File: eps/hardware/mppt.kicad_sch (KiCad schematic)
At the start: 16 parts, among them U2 LTC3130-1

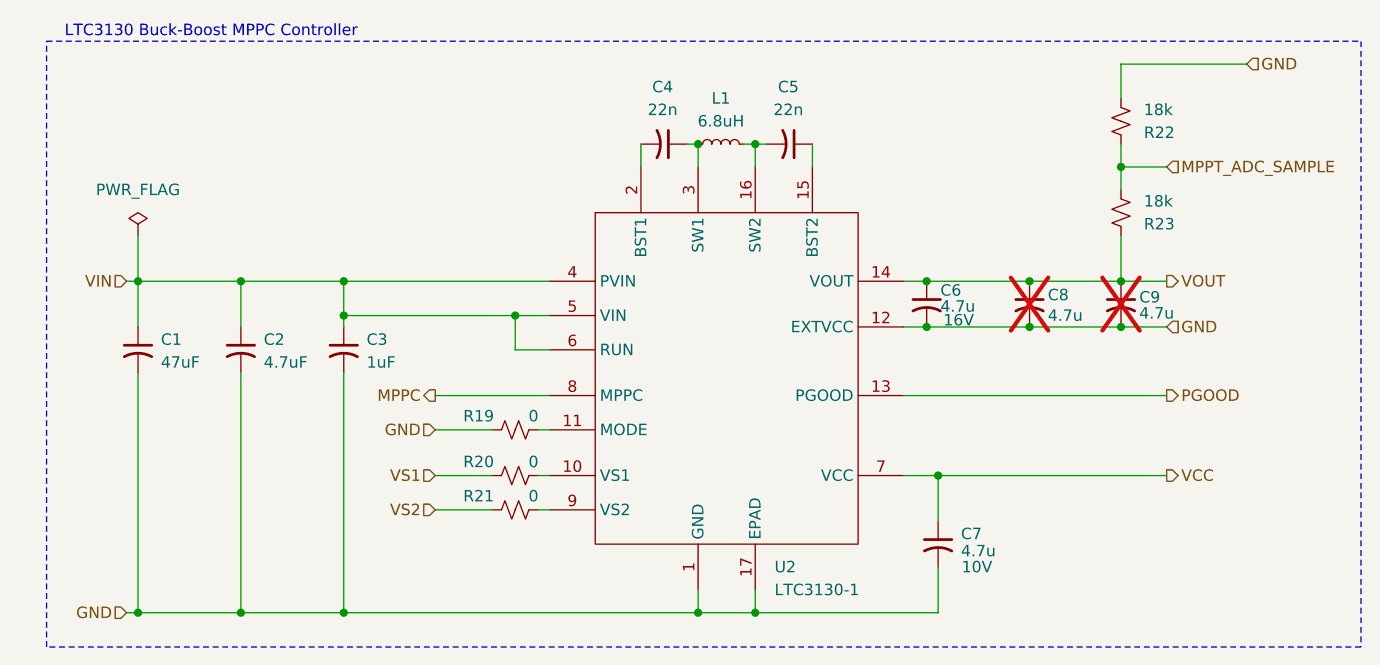
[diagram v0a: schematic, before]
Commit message: netlist fixes
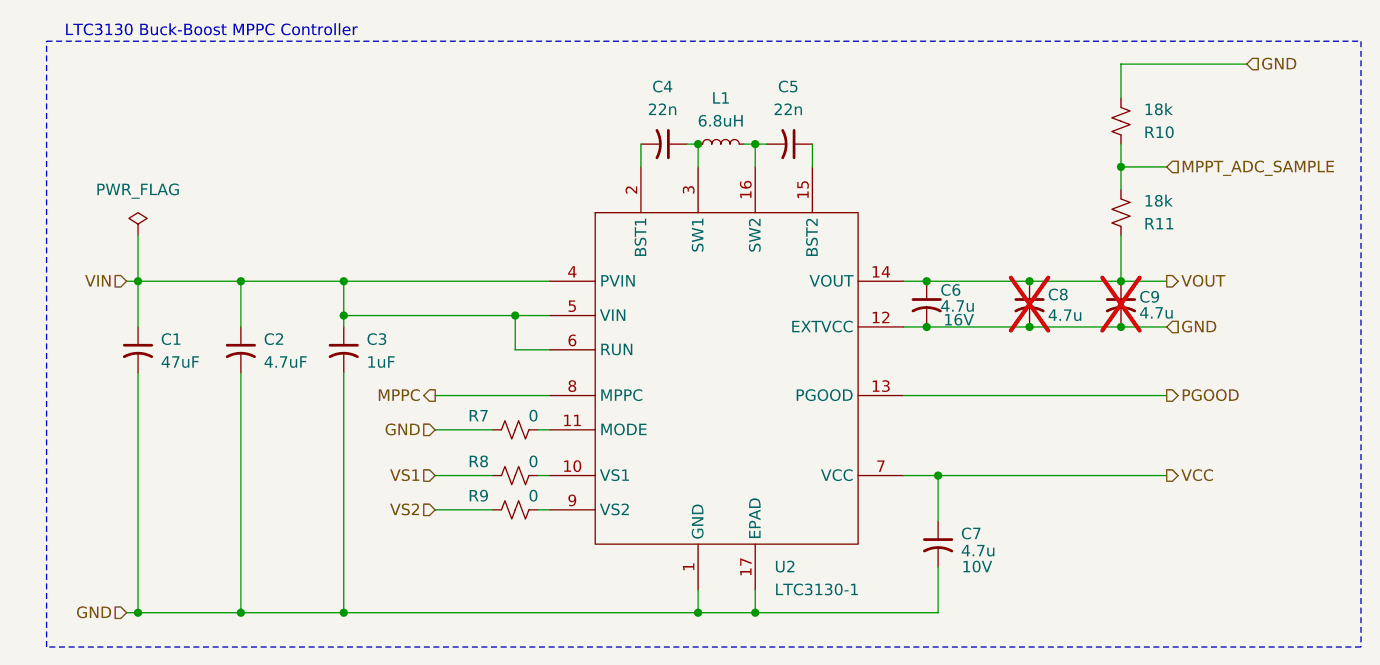
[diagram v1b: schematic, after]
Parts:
- renumbered R22 to R10, R23 to R11, R19 to R7, R20 to R8, R21 to R9
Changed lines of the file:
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@@
 		(on_board yes)
 		(dnp no)
-		(property "Reference" "R23"
+		(property "Reference" "R11"
 			(at 135.89 35.5601 0)
 			(effects
@@
 			(project "eps"
 				(path "/9e0ae2e7-d4be-41b4-8312-0d2aceea2180/fa2efaa0-4907-4b3e-94ec-ef462aa79480"
-					(reference "R23")
+					(reference "R11")
 					(unit 1)
 				)
@@
 		(on_board yes)
 		(dnp no)
-		(property "Reference" "R22"
+		(property "Reference" "R10"
 			(at 135.89 25.4001 0)
 			(effects
@@
 			(project "eps"
 				(path "/9e0ae2e7-d4be-41b4-8312-0d2aceea2180/fa2efaa0-4907-4b3e-94ec-ef462aa79480"
-					(reference "R22")
+					(reference "R10")
 					(unit 1)
 				)
@@
 		(on_board yes)
 		(dnp no)
-		(property "Reference" "R20"
+		(property "Reference" "R8"
 			(at 61.976 61.976 90)
 			(effects
@@
 			(project ""
 				(path "/9e0ae2e7-d4be-41b4-8312-0d2aceea2180/fa2efaa0-4907-4b3e-94ec-ef462aa79480"
-					(reference "R20")
+					(reference "R8")
 					(unit 1)
 				)
@@
 		(on_board yes)
 		(dnp no)
-		(property "Reference" "R21"
+		(property "Reference" "R9"
 			(at 61.976 65.786 90)
 			(effects
@@
 			(project "eps"
 				(path "/9e0ae2e7-d4be-41b4-8312-0d2aceea2180/fa2efaa0-4907-4b3e-94ec-ef462aa79480"
-					(reference "R21")
+					(reference "R9")
 					(unit 1)
 				)
@@
 		(on_board yes)
 		(dnp no)
-		(property "Reference" "R19"
+		(property "Reference" "R7"
 			(at 61.976 56.896 90)
 			(effects
@@
 			(project "eps"
 				(path "/9e0ae2e7-d4be-41b4-8312-0d2aceea2180/fa2efaa0-4907-4b3e-94ec-ef462aa79480"
-					(reference "R19")
+					(reference "R7")
 					(unit 1)
 				)
@@
 		(dnp no)
 		(fields_autoplaced yes)
-		(property "Reference" "#FLG02"
+		(property "Reference" "#FLG03"
 			(at 24.13 34.925 0)
 			(effects
@@
 			(project "eps"
 				(path "/9e0ae2e7-d4be-41b4-8312-0d2aceea2180/fa2efaa0-4907-4b3e-94ec-ef462aa79480"
-					(reference "#FLG02")
-					(unit 1)
-				)
+					(reference "#FLG03")
+					(unit 1)
+				)
